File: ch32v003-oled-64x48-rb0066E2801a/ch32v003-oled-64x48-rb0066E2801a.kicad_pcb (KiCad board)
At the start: 2 copper layers, 12.7 x 18.5 mm, 19 parts, among them J1 USB_C_Receptacle_USB2.0, J2 PGM, U1 CH32V003F4U6, U2 3.3vReg, U4 OLED-RB0066E2801A-64x48-FULL

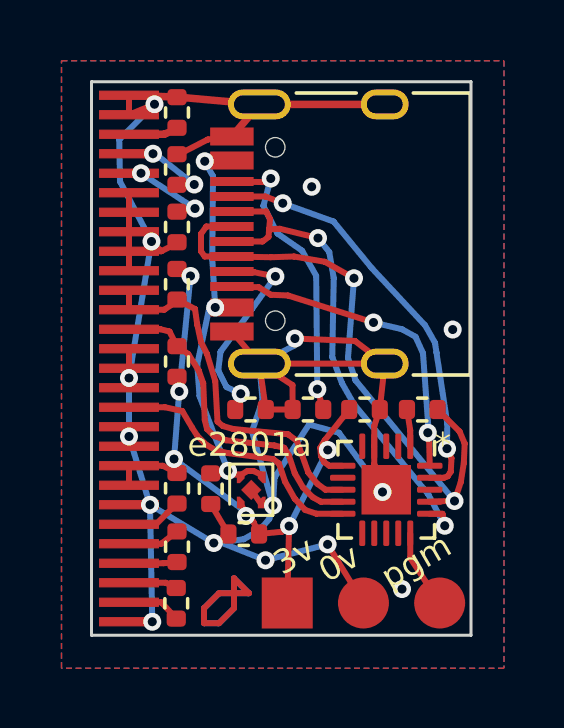
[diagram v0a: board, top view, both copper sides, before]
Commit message: Forgot to include the build files.
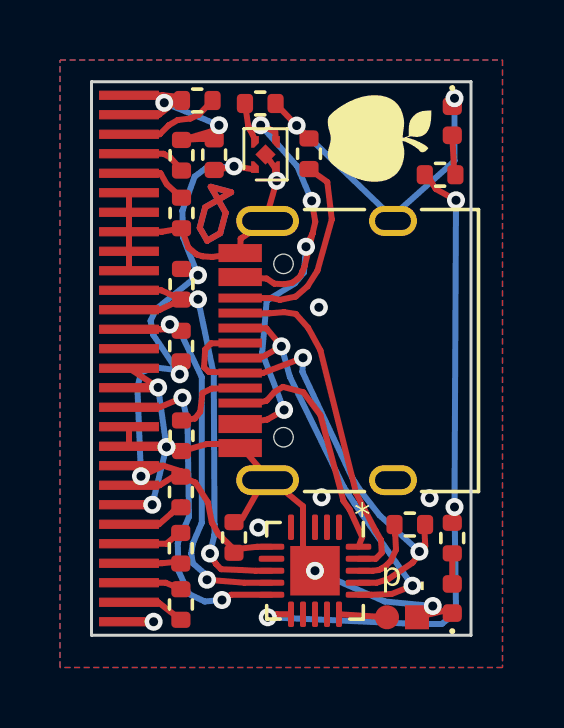
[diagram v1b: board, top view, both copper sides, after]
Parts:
- added D1: LED, LED_SMD:LED_0402_1005Metric, F.Cu at (114.0, 66.4)
- added D2: LED, LED_SMD:LED_0402_1005Metric, F.Cu at (114.0, 50.5)
- added J3: APPLE, artwork:apple, F.Cu at (111.6, 51.1)
- added R4: 10, Resistor_SMD:R_0402_1005Metric, F.Cu at (114.0, 64.4)
- added R5: 10, Resistor_SMD:R_0402_1005Metric, F.Cu at (113.6, 52.3)
- moved C2 12.9 mm to (107.6, 49.9), turned to 180 degrees
- moved U2 11.2 mm to (107.8, 51.6)
- moved C5 9.86 mm to (106.1, 51.6), turned to -90 degrees
- moved R3 8.53 mm to (109.2, 51.6), turned to 90 degrees
- moved J2 4.35 mm to (112.8, 67.0), turned to -90 degrees
- moved J1 3.89 mm to (111.0, 58.2)
- moved R1 3.86 mm to (112.6, 64.0)
- moved U1 3.60 mm to (109.5, 65.5)
- moved R2 2.46 mm to (105.0, 61.0), turned to -90 degrees
- moved C8 0.78 mm to (105.5, 49.8), turned to 0 degrees
- moved R10 0.53 mm to (105.0, 58.0)
- moved C3 0.50 mm to (105.0, 51.6)
- moved R11 0.49 mm to (105.0, 53.6)
- moved C1 0.34 mm to (106.8, 64.4), turned to -90 degrees
- moved R12 0.18 mm to (105.0, 62.9)
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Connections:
- J2 pad 1: VDD -> GND
- J2 pad 2: GND -> PGM
- R1 pad 2: Net-(R1-Pad2) -> Net-(U1-Pad18)
- U1 pad 1: Net-(R1-Pad2) -> unconnected-(U1-Pad1)
- U1 pad 18: unconnected-(U1-Pad18) -> Net-(U1-Pad18)
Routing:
- net GND: track 84.8 -> 54.8 mm
- net FIOB: track 0.00 -> 23.0 mm, vias 0 -> 3
- net +5V: track 13.6 -> 18.7 mm, vias 3 -> 4
- net Net-(J1-PadA5): track 6.90 -> 2.58 mm, vias 2 -> 0
- net RES: track 8.80 -> 12.3 mm, vias 0 -> 2
- net D-: track 20.3 -> 16.8 mm
- net SCL: track 10.7 -> 13.8 mm, vias 0 -> 2
- net Net-(J1-PadB5): track 9.90 -> 6.84 mm, vias 2 -> 0
- net SBU2: track 10.8 -> 7.99 mm, vias 2 -> 0
- net SDA: track 12.3 -> 15.1 mm, vias 0 -> 2
- net SBU1: track 14.0 -> 11.3 mm, vias 2 -> 0
- net Net-(U1-Pad18): track 0.00 -> 2.52 mm
- net D+: track 16.7 -> 14.2 mm
- net VDD: track 23.7 -> 25.3 mm, vias 6 -> 4
- net Net-(C8-Pad2): track 1.72 -> 3.19 mm
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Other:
- board text added: "-"
- board text added: "p"
- board text removed: "0v"
- board text removed: "3v"
- board text removed: "e2801a"
- board text removed: "pgm"
